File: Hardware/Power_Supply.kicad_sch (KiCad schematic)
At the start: 20 parts, among them J2 Screw_Terminal_01x02, U11 B0505S, U3 XL1509-5.0, U9 LD1117

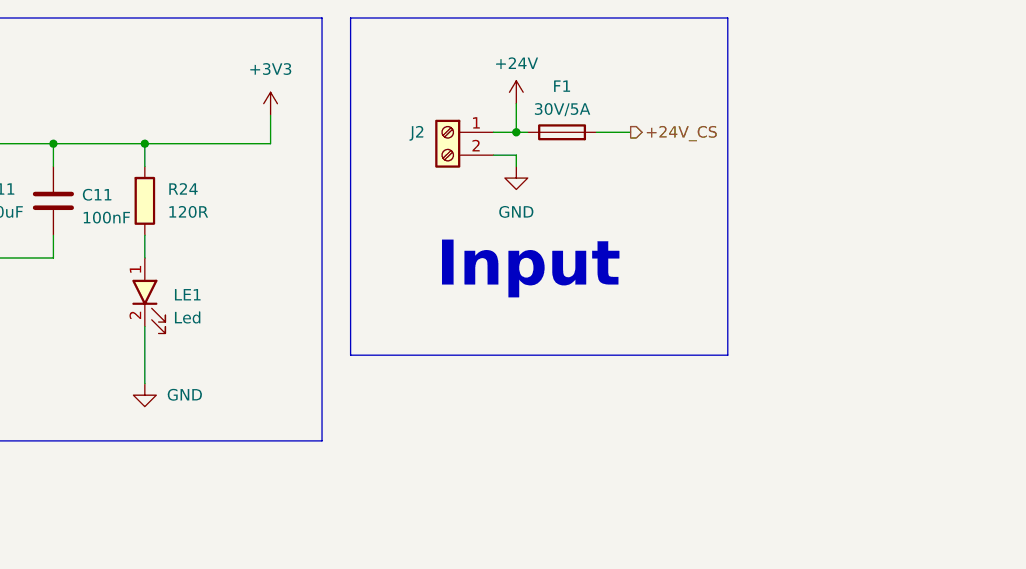
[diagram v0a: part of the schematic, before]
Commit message: Layout track part 2
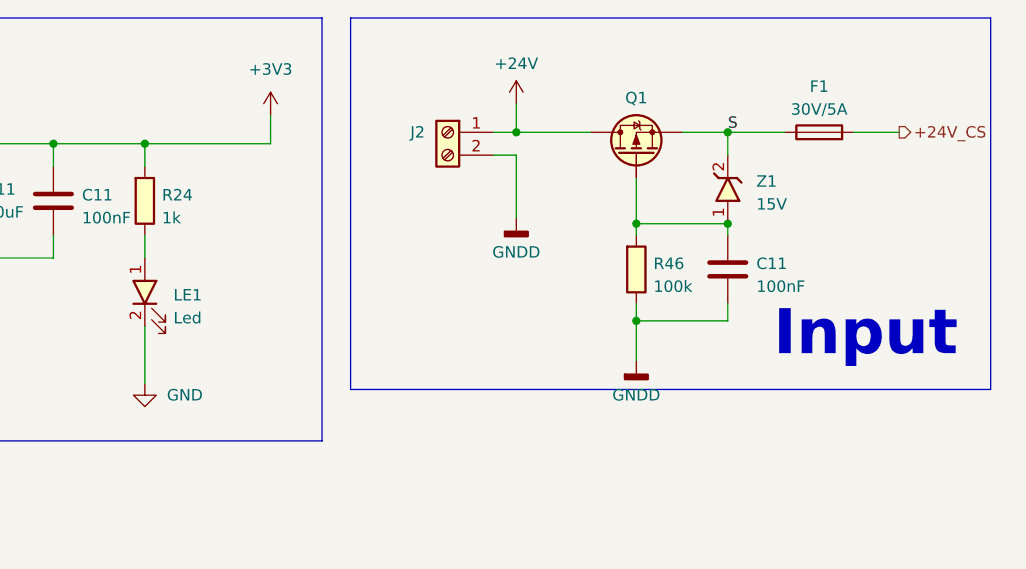
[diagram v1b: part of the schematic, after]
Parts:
- added C11: 100nF, IVS_FOOTPRINTS:C_0603, symbol IVS_SYMBOLS:C
- added Q1: P_Mosfet, Package_TO_SOT_SMD:TO-252-2, symbol IVS_SYMBOLS:P_Mosfet_1G2D3S
- added R46: 100k, IVS_FOOTPRINTS:R_0603, symbol IVS_SYMBOLS:R
- added Z1: 15V, IVS_FOOTPRINTS:Package-Diode-D_MiniMELF, symbol IVS_SYMBOLS:D_Zener
- C15: footprint IVS_FOOTPRINTS:C_0603 -> IVS_FOOTPRINTS:C_1206
- R24: value 120R -> 1k
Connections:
- net +24V: now also Q1.2 (D); no longer F1.1
- net GND: no longer J2.2 (Pin_2)
- net GNDD: now also J2.2 (Pin_2), C11.2, R46.2
- new net: C11.1, Q1.1 (G), R46.1, Z1.1
- new net S: F1.1, Q1.3 (S), Z1.2
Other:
- moved on the sheet: F1
